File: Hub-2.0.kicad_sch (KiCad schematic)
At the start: 5 parts, among them CN1 DT15-12PA, CN2 DT15-12PA, SW1 SW_Push_Open, SW2 SW_Push_Open

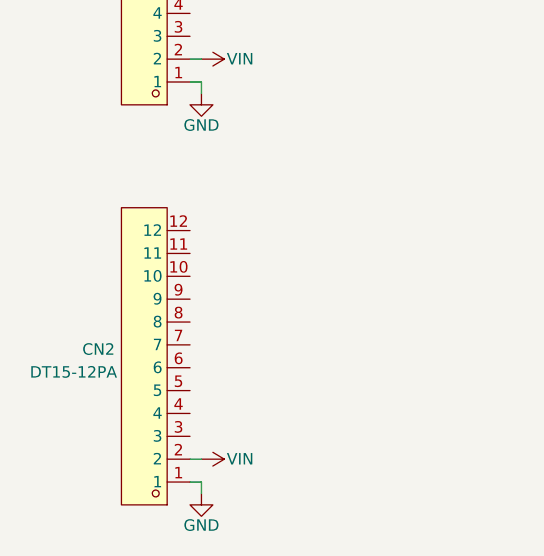
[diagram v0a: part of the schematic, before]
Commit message: Autosave
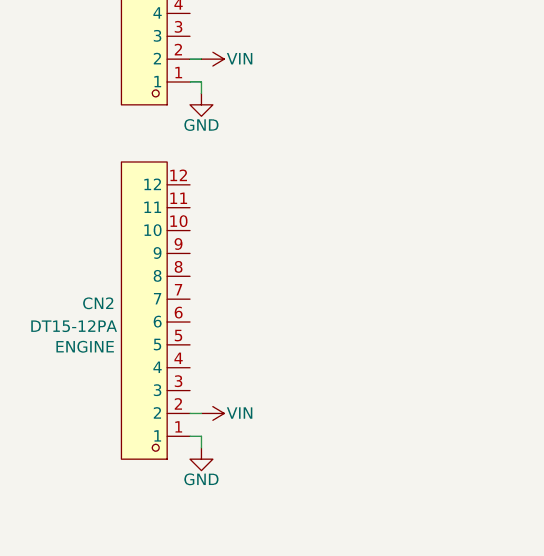
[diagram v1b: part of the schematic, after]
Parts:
- CN2: Name (none) -> ENGINE
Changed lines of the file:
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@@
 	(wire
 		(pts
-			(xy 74.93 87.63) (xy 74.93 86.36)
+			(xy 74.93 127) (xy 74.93 125.73)
 		)
 		(stroke
@@
 	(wire
 		(pts
-			(xy 73.66 128.27) (xy 74.93 128.27)
+			(xy 74.93 87.63) (xy 74.93 86.36)
 		)
 		(stroke
@@
 	(wire
 		(pts
-			(xy 74.93 132.08) (xy 74.93 130.81)
+			(xy 247.65 26.67) (xy 248.92 26.67)
 		)
 		(stroke
@@
 	(wire
 		(pts
-			(xy 247.65 26.67) (xy 248.92 26.67)
+			(xy 215.9 26.67) (xy 242.57 26.67)
 		)
 		(stroke
@@
 	(wire
 		(pts
-			(xy 215.9 26.67) (xy 242.57 26.67)
+			(xy 73.66 123.19) (xy 74.93 123.19)
 		)
 		(stroke
@@
 	(wire
 		(pts
-			(xy 74.93 130.81) (xy 73.66 130.81)
+			(xy 74.93 125.73) (xy 73.66 125.73)
 		)
 		(stroke
@@
 	)
 	(symbol
-		(lib_id "power:GND")
-		(at 74.93 132.08 0)
+		(lib_id "EasyEDA:DT15-12PA")
+		(at 69.85 111.76 180)
 		(unit 1)
 		(body_style 1)
@@
 		(in_pos_files yes)
 		(dnp no)
-		(property "Reference" "#PWR04"
-			(at 74.93 138.43 0)
+		(property "Reference" "CN2"
+			(at 63.5 110.998 0)
+			(show_name no)
+			(do_not_autoplace no)
+			(effects
+				(font
+					(size 1.27 1.27)
+				)
+			)
+		)
+		(property "Value" "DT15-12PA"
+			(at 60.706 113.538 0)
+			(show_name no)
+			(do_not_autoplace no)
+			(effects
+				(font
+					(size 1.27 1.27)
+				)
+			)
+		)
+		(property "Footprint" "EasyEDA:CONN-TH_DT15-12PA"
+			(at 69.85 90.17 0)
 			(hide yes)
 			(show_name no)
@@
 			)
 		)
-		(property "Value" "GND"
-			(at 74.93 135.636 0)
+		(property "Datasheet" "https://www.lcsc.com/datasheet/C5341788.pdf"
+			(at 69.85 87.63 0)
+			(hide yes)
 			(show_name no)
 			(do_not_autoplace no)
@@
 			)
 		)
-		(property "Footprint" ""
-			(at 74.93 132.08 0)
+		(property "Description" ""
+			(at 69.85 111.76 0)
 			(hide yes)
 			(show_name no)
@@
 			)
 		)
-		(property "Datasheet" ""
-			(at 74.93 132.08 0)
+		(property "Manufacturer" "TE Connectivity(泰科电子)"
+			(at 69.85 85.09 0)
 			(hide yes)
 			(show_name no)
@@
 			)
 		)
-		(property "Description" "Power symbol creates a global label with name \"GND\" , ground"
-			(at 74.93 132.08 0)
+		(property "MPN" "DT15-12PA"
+			(at 69.85 82.55 0)
 			(hide yes)
 			(show_name no)
@@
 			)
 		)
+		(property "LCSC Part" "C5341788"
+			(at 69.85 80.01 0)
+			(hide yes)
+			(show_name no)
+			(do_not_autoplace no)
+			(effects
+				(font
+					(size 1.27 1.27)
+				)
+			)
+		)
+		(property "Name" "ENGINE"
+			(at 61.976 115.824 0)
+			(show_name no)
+			(do_not_autoplace no)
+			(effects
+				(font
+					(size 1.27 1.27)
+				)
+			)
+		)
+		(pin "10"
+		)
+		(pin "8"
+		)
+		(pin "12"
+		)
+		(pin "9"
+		)
+		(pin "11"
+		)
+		(pin "5"
+		)
+		(pin "7"
+		)
+		(pin "6"
+		)
+		(pin "3"
+		)
+		(pin "2"
+		)
+		(pin "4"
+		)
 		(pin "1"
 		)
@@
 			(project "Hub-2.0"
 				(path "/af8ad92e-80c5-47c7-b528-865d82af0364"
-					(reference "#PWR04")
+					(reference "CN2")
 					(unit 1)
 				)
@@
 	)
 	(symbol
-		(lib_id "EasyEDA:DT15-12PA")
-		(at 69.85 116.84 180)
+		(lib_id "power:+5V")
+		(at 74.93 123.19 270)
 		(unit 1)
 		(body_style 1)
@@
 		(in_pos_files yes)
 		(dnp no)
-		(property "Reference" "CN2"
-			(at 63.5 116.078 0)
-			(show_name no)
-			(do_not_autoplace no)
-			(effects
-				(font
-					(size 1.27 1.27)
-				)
-			)
-		)
-		(property "Value" "DT15-12PA"
-			(at 60.706 118.618 0)
-			(show_name no)
-			(do_not_autoplace no)
-			(effects
-				(font
-					(size 1.27 1.27)
-				)
-			)
-		)
-		(property "Footprint" "EasyEDA:CONN-TH_DT15-12PA"
-			(at 69.85 95.25 0)
-			(hide yes)
-			(show_name no)
-			(do_not_autoplace no)
-			(effects
-				(font
-					(size 1.27 1.27)
-				)
-			)
-		)
-		(property "Datasheet" "https://www.lcsc.com/datasheet/C5341788.pdf"
-			(at 69.85 92.71 0)
+		(property "Reference" "#PWR03"
+			(at 71.12 123.19 0)
 			(hide yes)
 			(show_name no)
@@
 			)
 		)
-		(property "Description" ""
-			(at 69.85 116.84 0)
-			(hide yes)
+		(property "Value" "VIN"
+			(at 79.248 123.19 90)
 			(show_name no)
 			(do_not_autoplace no)
@@
 			)
 		)
-		(property "Manufacturer" "TE Connectivity(泰科电子)"
-			(at 69.85 90.17 0)
+		(property "Footprint" ""
+			(at 74.93 123.19 0)
 			(hide yes)
 			(show_name no)
@@
 			)
 		)
-		(property "MPN" "DT15-12PA"
-			(at 69.85 87.63 0)
+		(property "Datasheet" ""
+			(at 74.93 123.19 0)
 			(hide yes)
 			(show_name no)
@@
 			)
 		)
-		(property "LCSC Part" "C5341788"
-			(at 69.85 85.09 0)
+		(property "Description" "Power symbol creates a global label with name \"+5V\""
+			(at 74.93 123.19 0)
 			(hide yes)
 			(show_name no)
@@
 			)
 		)
-		(pin "10"
-		)
-		(pin "8"
-		)
-		(pin "12"
-		)
-		(pin "9"
-		)
-		(pin "11"
-		)
-		(pin "5"
-		)
-		(pin "7"
-		)
-		(pin "6"
-		)
-		(pin "3"
-		)
-		(pin "2"
-		)
-		(pin "4"
-		)
 		(pin "1"
 		)
@@
 			(project "Hub-2.0"
 				(path "/af8ad92e-80c5-47c7-b528-865d82af0364"
-					(reference "CN2")
+					(reference "#PWR03")
 					(unit 1)
 				)
@@
 	)
 	(symbol
-		(lib_id "power:+5V")
-		(at 74.93 128.27 270)
+		(lib_id "power:GND")
+		(at 74.93 127 0)
 		(unit 1)
 		(body_style 1)
@@
 		(in_pos_files yes)
 		(dnp no)
-		(property "Reference" "#PWR03"
-			(at 71.12 128.27 0)
+		(property "Reference" "#PWR04"
+			(at 74.93 133.35 0)
 			(hide yes)
 			(show_name no)
@@
 			)
 		)
-		(property "Value" "VIN"
-			(at 79.248 128.27 90)
+		(property "Value" "GND"
+			(at 74.93 130.556 0)
 			(show_name no)
 			(do_not_autoplace no)
@@
 		)
 		(property "Footprint" ""
-			(at 74.93 128.27 0)
+			(at 74.93 127 0)
 			(hide yes)
 			(show_name no)
@@
 		)
 		(property "Datasheet" ""
-			(at 74.93 128.27 0)
+			(at 74.93 127 0)
 			(hide yes)
 			(show_name no)
@@
 			)
 		)
-		(property "Description" "Power symbol creates a global label with name \"+5V\""
-			(at 74.93 128.27 0)
+		(property "Description" "Power symbol creates a global label with name \"GND\" , ground"
+			(at 74.93 127 0)
 			(hide yes)
 			(show_name no)
@@
 			(project "Hub-2.0"
 				(path "/af8ad92e-80c5-47c7-b528-865d82af0364"
-					(reference "#PWR03")
+					(reference "#PWR04")
 					(unit 1)
 				)
